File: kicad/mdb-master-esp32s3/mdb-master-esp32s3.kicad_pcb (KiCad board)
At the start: 2 copper layers, 41.8 x 53.2 mm, 37 parts, among them J1 Conn_02x09_Odd_Even, J2 MDB_Connector, J3 Barrel_Jack, P1 USB_C_Plug_USB2.0, Q1 BC807, U1 ESP32-S3, U2 LM317_SOT-223, Y1 Crystal

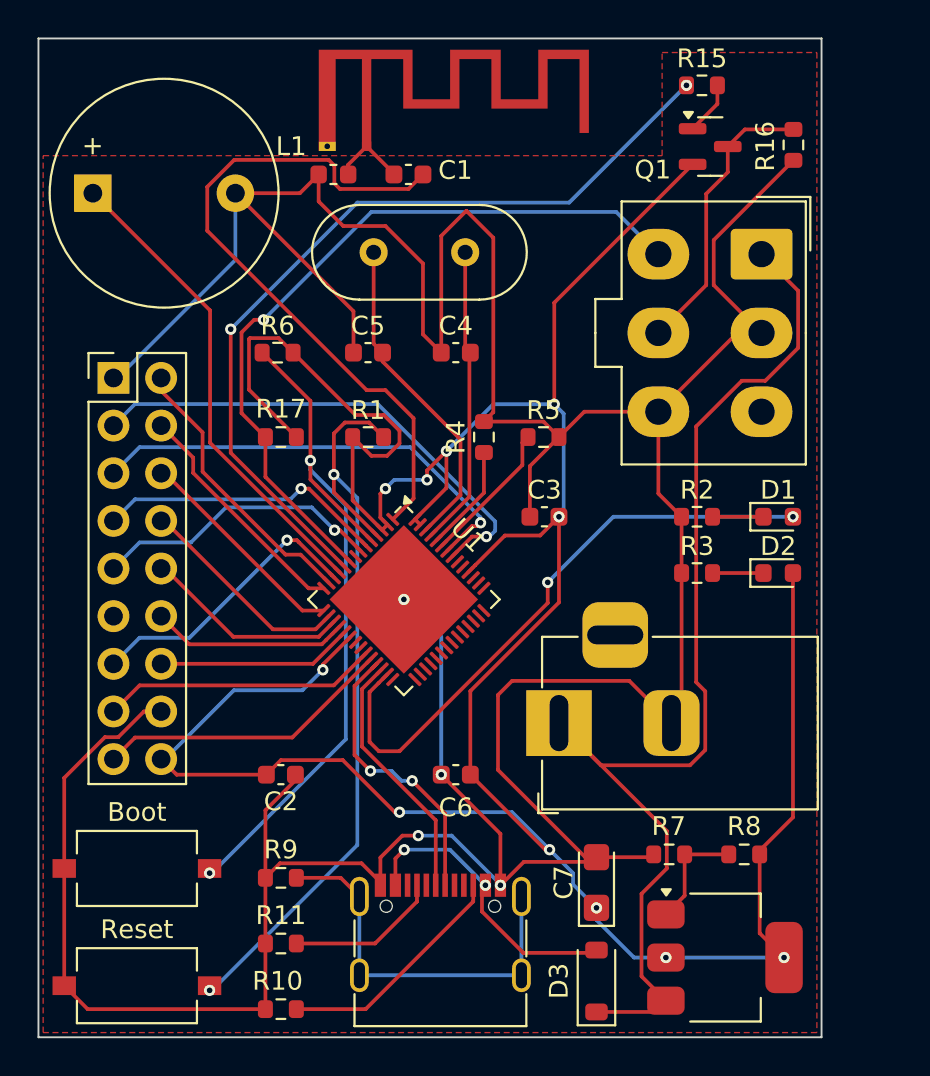
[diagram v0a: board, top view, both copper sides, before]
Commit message: refacting
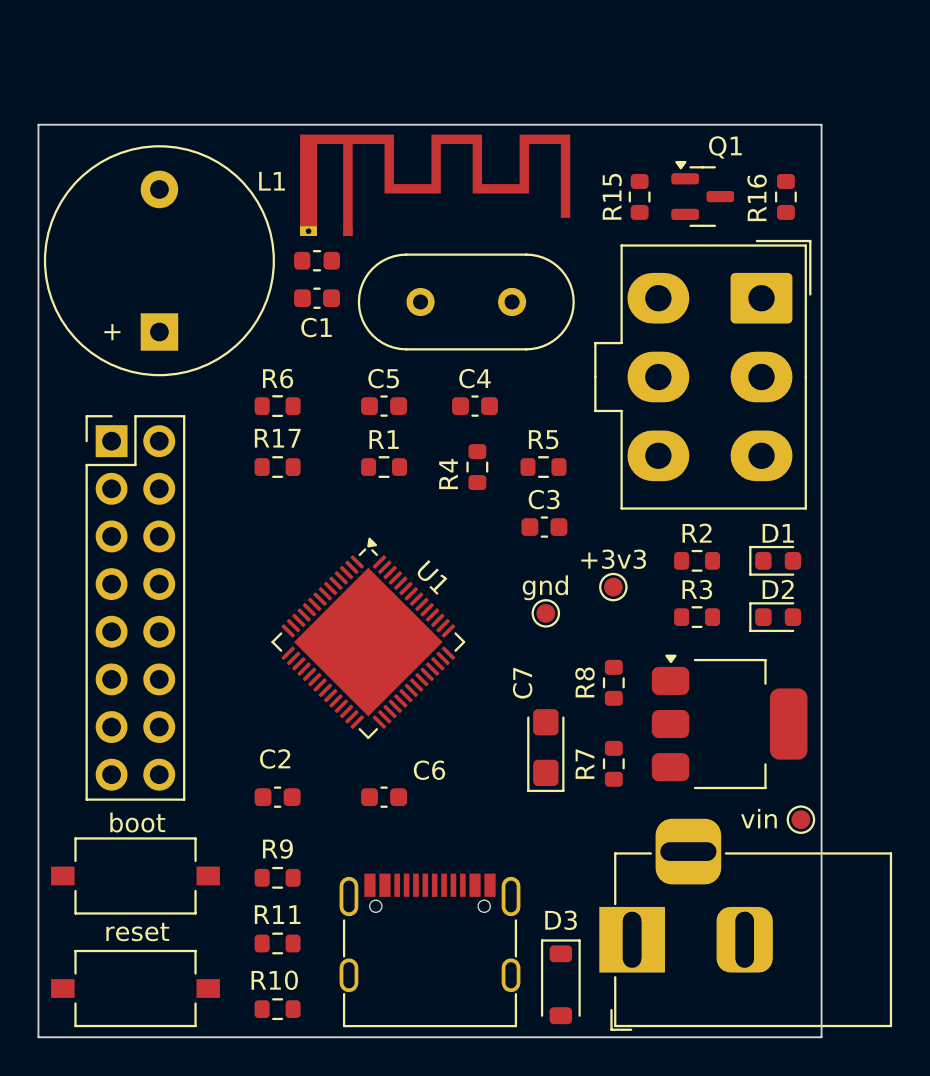
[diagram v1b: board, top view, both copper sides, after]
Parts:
- removed Boot: Boot, Button_Switch_SMD:SW_Tactile_SPST_NO_Straight_CK_PTS636Sx25SMTRLFS
- removed J1: Conn_02x09_Odd_Even, Connector_PinHeader_2.54mm:PinHeader_2x09_P2.54mm_Vertical
- removed Reset: Reset, Button_Switch_SMD:SW_Tactile_SPST_NO_Straight_CK_PTS636Sx25SMTRLFS
- added +3v3: TestPoint, TestPoint:TestPoint_Pad_D1.0mm, F.Cu at (152.4, 117.0)
- added J4: Conn_02x08_Odd_Even, Connector_PinHeader_2.54mm:PinHeader_2x08_P2.54mm_Vertical, F.Cu at (125.7, 109.2)
- added boot: Boot, Button_Switch_SMD:SW_Tactile_SPST_NO_Straight_CK_PTS636Sx25SMTRLFS, F.Cu at (126.9, 132.4)
- added gnd: TestPoint, TestPoint:TestPoint_Pad_D1.0mm, F.Cu at (148.8, 118.4)
- added reset: Reset, Button_Switch_SMD:SW_Tactile_SPST_NO_Straight_CK_PTS636Sx25SMTRLFS, F.Cu at (126.9, 138.4)
- added vin: TestPoint, TestPoint:TestPoint_Pad_D1.0mm, F.Cu at (162.4, 129.4)
- moved U2 12.5 mm to (158.6, 124.3)
- moved J3 12.2 mm to (153.4, 135.8)
- moved R8 11.5 mm to (152.4, 122.1), turned to -90 degrees
- moved BZ1 8.21 mm to (128.2, 103.4), turned to 90 degrees
- moved C1 8.21 mm to (136.6, 101.6), turned to 180 degrees
- moved C7 7.68 mm to (148.8, 125.6)
- moved R15 6.81 mm to (153.8, 96.2), turned to 90 degrees
- moved R7 5.66 mm to (152.4, 126.4), turned to -90 degrees
- moved L1 4.68 mm to (136.6, 99.6)
- moved AE1 4.63 mm to (138.2, 98.0)
- moved C6 4.01 mm to (140.2, 128.2)
- moved Y1 3.64 mm to (142.1, 101.8)
- moved C4 3.03 mm to (145.0, 107.3)
- moved C5 2.98 mm to (140.2, 107.3)
- moved U1 2.96 mm to (139.3, 119.9)
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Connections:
- net +36V renamed /vin
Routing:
- net GND: track 220.5 -> 0.00 mm, vias 4 -> 0
- net +3V3: track 167.8 -> 0.00 mm, vias 11 -> 0
- net /vin: track 61.7 -> 0.00 mm
- net /io5: track 44.9 -> 0.00 mm, vias 2 -> 0
- net Net-(U1-CHIP_PU/RESET): track 40.8 -> 0.00 mm, vias 2 -> 0
- net /io4: track 40.4 -> 0.00 mm, vias 1 -> 0
- net /boot: track 38.2 -> 0.00 mm, vias 2 -> 0
- net Net-(U1-LNA_IN/RF): track 36.9 -> 0.00 mm
- net /io21: track 32.6 -> 0.00 mm, vias 2 -> 0
- net /u0txd: track 26.8 -> 0.00 mm, vias 1 -> 0
- net /io6: track 25.7 -> 0.00 mm
- net /u0rxd: track 24.4 -> 0.00 mm, vias 1 -> 0
- net Net-(P1-SHIELD): track 20.8 -> 0.00 mm
- net Net-(U1-XTAL_P): track 17.5 -> 0.00 mm
- net Net-(U1-XTAL_N): track 16.1 -> 0.00 mm
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- removed copper zone on F.Cu, net GND
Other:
- board size 41.8 x 53.2 mm -> 41.8 x 48.7 mm
